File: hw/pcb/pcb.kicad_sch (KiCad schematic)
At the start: 66 parts, among them J1 ConnMain, J2 ConnPorts, J3 Conn_01x01_Pin, J4 Conn_01x01_Pin, J5 Conn_01x01_Pin, J6 Conn_01x01_Pin

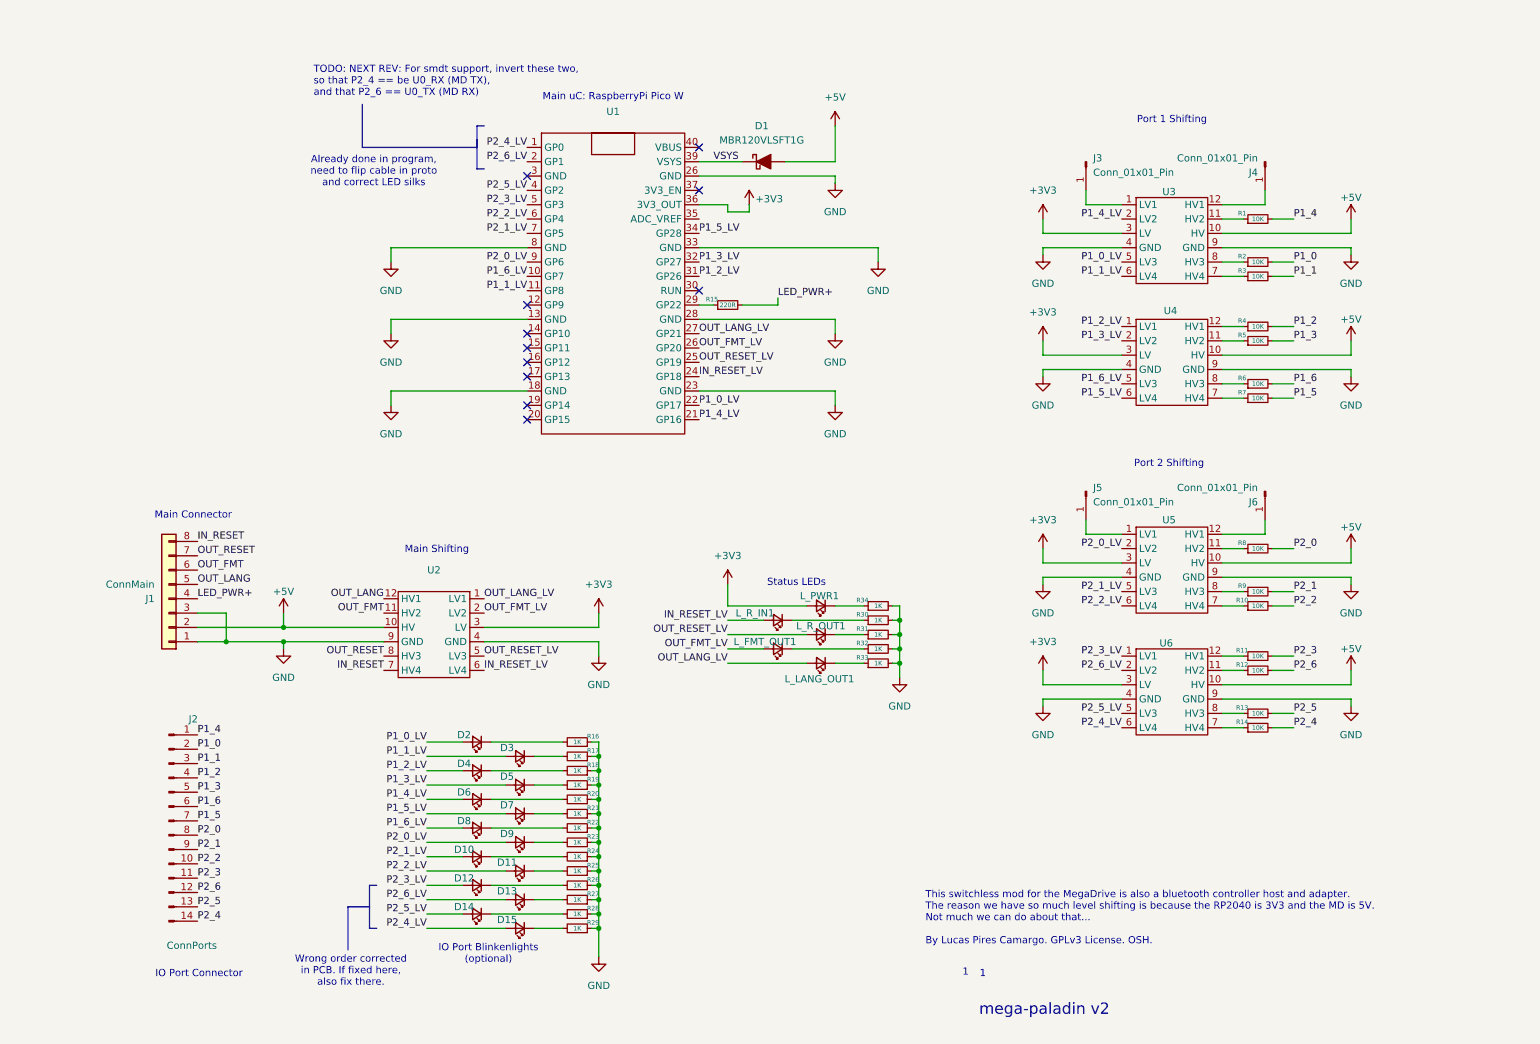
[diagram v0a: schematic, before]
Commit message: [hw] initial v3 design, updated readme
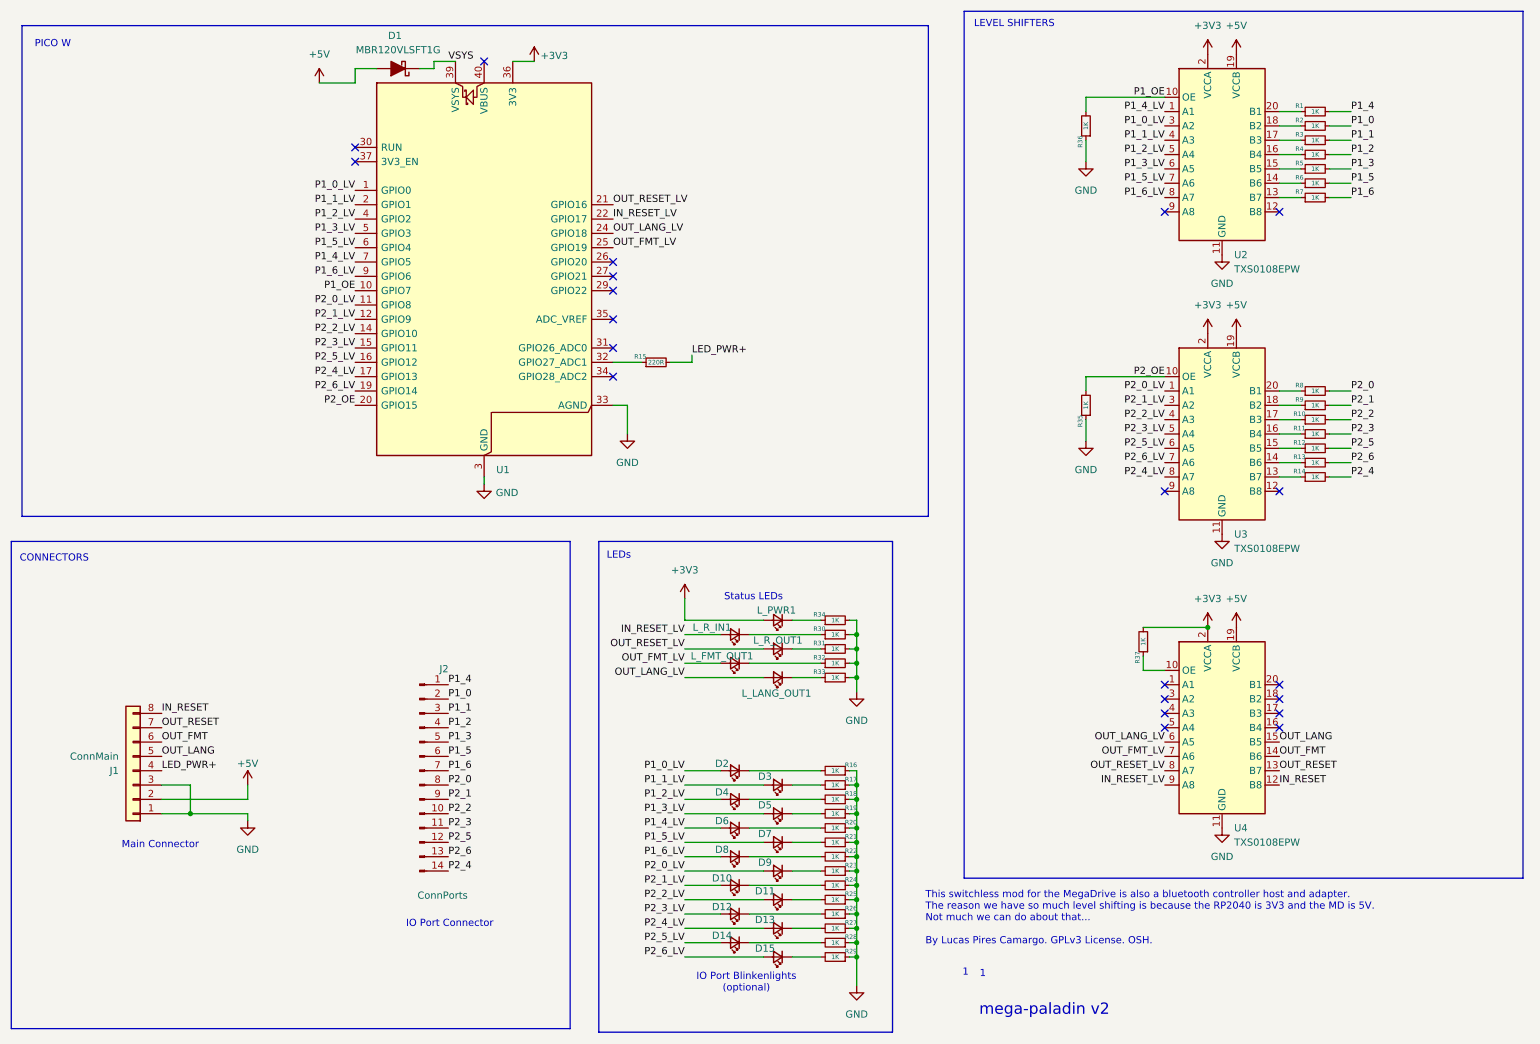
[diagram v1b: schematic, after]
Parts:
- removed J3, J4, J5, J6: Conn_01x01_Pin, Connector_PinHeader_2.54mm:PinHeader_1x01_P2.54mm_Vertical, symbol Connector:Conn_01x01_Pin
- removed U2, U3, U4, U5, U6: ~, footprints:cheap_lvl_shifter_4ch, symbol modules:lvl_shifter
- added R35, R36, R37: 1K, Resistor_SMD:R_0805_2012Metric_Pad1.20x1.40mm_HandSolder, symbol Device:R_Small
- added U2, U3, U4: TXS0108EPW, Package_SO:TSSOP-20_4.4x6.5mm_P0.65mm, symbol Logic_LevelTranslator:TXS0108EPW
- J2: footprint Connector_PinHeader_2.54mm:PinHeader_1x14_P2.54mm_Horizontal -> Connector_PinHeader_2.54mm:PinHeader_1x14_P2.54mm_Vertical
- R1, R10, R11, R12, R13, R14, R2, R3, R4, R5, R6, R7, R8, R9: value 10K -> 1K
- U1: footprint Module_RaspberryPi_Pico:RaspberryPi_Pico_W_SMD_MountingHoles_Castellated_HandSolder -> Module:RaspberryPi_Pico_W_SMD_HandSolder; symbol modules:pico_w -> MCU_Module:RaspberryPi_Pico_W
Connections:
- net +3V3: now also R37.2, U2.2 (VCCA), U3.2 (VCCA), U4.2 (VCCA)
- net +5V: now also U2.19 (VCCB), U3.19 (VCCB), U4.19 (VCCB)
- net GND: now also U1.3 (GND), U1.38 (GND), R35.1, R36.1, U2.11 (GND), U3.11 (GND), U4.11 (GND); no longer U1.26 (GP20)
- net IN_RESET: now also U4.12 (B8)
- net IN_RESET_LV: now also U1.22 (GPIO17), U4.9 (A8); no longer U1.24 (GP18)
- net OUT_FMT: now also U4.14 (B6)
- net OUT_FMT_LV: now also U1.25 (GPIO19), U4.7 (A6); no longer U1.26 (GP20)
- net OUT_LANG: now also U4.15 (B5)
- net OUT_LANG_LV: now also U1.24 (GPIO18), U4.6 (A5); no longer U1.27 (GP21)
- net OUT_RESET: now also U4.13 (B7)
- net OUT_RESET_LV: now also U1.21 (GPIO16), U4.8 (A7); no longer U1.25 (GP19)
- net P1_0_LV: now also U1.1 (GPIO0), U2.3 (A2); no longer U1.22 (GP17)
- net P1_1_LV: now also U1.2 (GPIO1), U2.4 (A3); no longer U1.11 (GP8)
- net P1_2_LV: now also U1.4 (GPIO2), U2.5 (A4); no longer U1.31 (GP26)
- net P1_3_LV: now also U1.5 (GPIO3), U2.6 (A5); no longer U1.32 (GP27)
- net P1_4_LV: now also U1.7 (GPIO5), U2.1 (A1); no longer U1.21 (GP16)
- net P1_5: now also J2.6 (Pin_6), R6.2; no longer J2.7 (Pin_7), R7.2
- net P1_5_LV: now also U1.6 (GPIO4), U2.7 (A6); no longer U1.34 (GP28)
- net P1_6: now also J2.7 (Pin_7), R7.2; no longer J2.6 (Pin_6), R6.2
- net P1_6_LV: now also U1.9 (GPIO6), U2.8 (A7); no longer U1.10 (GP7)
- net P2_0_LV: now also U1.11 (GPIO8), U3.1 (A1); no longer U1.9 (GP6)
- net P2_1_LV: now also U1.12 (GPIO9), U3.3 (A2); no longer U1.7 (GP5)
- net P2_2_LV: now also U1.14 (GPIO10), U3.4 (A3); no longer U1.6 (GP4)
- net P2_3_LV: now also U1.15 (GPIO11), U3.5 (A4); no longer U1.5 (GP3)
- net P2_4_LV: now also D13.2 (A), U1.17 (GPIO13), U3.8 (A7); no longer D15.2 (A), U1.1 (GP0)
- net P2_5: now also J2.12 (Pin_12), R12.2; no longer J2.13 (Pin_13), R13.2
- net P2_5_LV: now also U1.16 (GPIO12), U3.6 (A5); no longer U1.4 (GP2)
- net P2_6: now also J2.13 (Pin_13), R13.2; no longer J2.12 (Pin_12), R12.2
- net P2_6_LV: now also D15.2 (A), U1.19 (GPIO14), U3.7 (A6); no longer D13.2 (A), U1.2 (GP1)
- net at R6.1: now also U2.14 (B6)
- net at R8.1: now also U3.20 (B1)
- net at R12.1: now also U3.15 (B5)
- net at R10.1: now also U3.17 (B3)
- net at R9.1: now also U3.18 (B2)
- net at R7.1: now also U2.13 (B7)
- net at R14.1: now also U3.13 (B7)
- net at R4.1: now also U2.16 (B4)
- net at R5.1: now also U2.15 (B5)
- net at R3.1: now also U2.17 (B3)
- net at R15.1: now also U1.32 (GPIO27_ADC1); no longer U1.29 (GP22)
- net at R13.1: now also U3.14 (B6)
- net at R11.1: now also U3.16 (B4)
- net at R1.1: now also U2.20 (B1)
- net at R2.1: now also U2.18 (B2)
- net P2_OE: now reaches U1.20 (GPIO15)
- net P2_OE: now also R35.2, U3.10 (OE)
- new net: R37.1, U4.10 (OE)
- new net P1_OE: R36.2, U1.10 (GPIO7), U2.10 (OE)
- no-connect marks 11 -> 21
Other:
- note added: "CONNECTORS"
- note added: "LEDs"
- note added: "LEVEL SHIFTERS"
- note added: "PICO W"
- note removed: "Already done in program, need to flip cable in proto and correct LED silks"
- note removed: "Main Shifting"
- note removed: "Main uC: RaspberryPi Pico W"
- note removed: "Port 1 Shifting"
- note removed: "Port 2 Shifting"
- note removed: "TODO: NEXT REV: For smdt support, invert these two, so that P2_4 == be U0_RX (MD TX), and that P2_6 == U0_TX (MD RX)"
- note removed: "Wrong order corrected in PCB. If fixed here, also fix there."
- moved on the sheet: D1, D10, D11, D12, D13, D14, D15, D2, D3, D4, D5, D6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
